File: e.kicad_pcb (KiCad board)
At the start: 2 copper layers, 69.8 x 81.6 mm, 8 parts, among them SW1 SW_Push, SW2 SW_Push, U2 MAX98357A

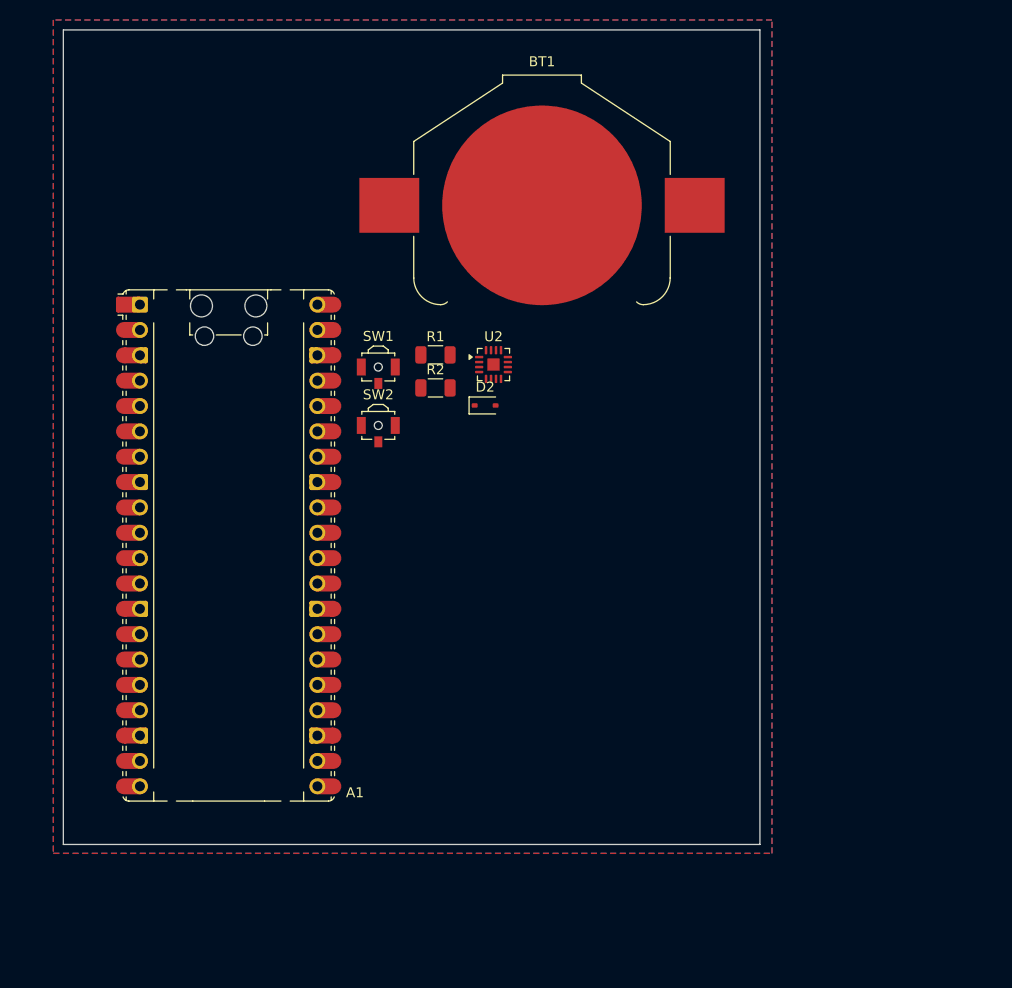
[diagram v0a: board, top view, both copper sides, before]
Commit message: i did MORE things
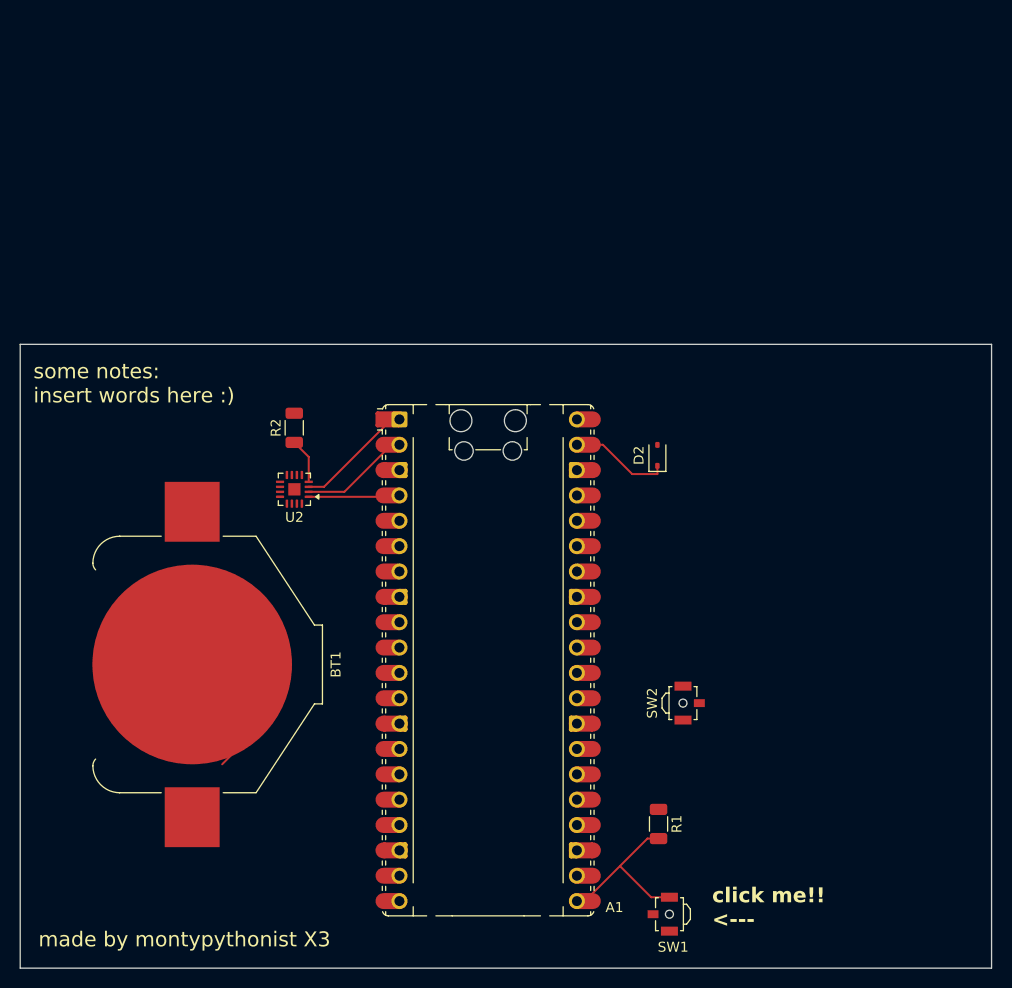
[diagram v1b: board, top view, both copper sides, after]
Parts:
- SW1: value SW_Push -> pwr
- SW2: value SW_Push -> rst
- moved SW1 61.0 mm to (159.9, 137.1), turned to -90 degrees
- moved BT1 57.8 mm to (112.9, 112.1), turned to -90 degrees
- moved R1 52.0 mm to (159.6, 128.1), turned to -90 degrees
- moved SW2 41.4 mm to (162.9, 115.9), turned to 90 degrees
- moved A1 28.4 mm to (142.6, 111.7)
- moved U2 23.5 mm to (123.2, 94.5), turned to 180 degrees
- moved D2 18.0 mm to (159.5, 91.1), turned to 90 degrees
- moved R2 14.7 mm to (123.1, 88.4), turned to 90 degrees
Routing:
- net Net-(A1-GPIO16): track 0.00 -> 16.2 mm
- net Net-(A1-GPIO0): track 0.00 -> 11.1 mm
- net Net-(A1-GPIO1): track 0.00 -> 10.2 mm
- net Net-(A1-VSYS): track 0.00 -> 9.30 mm
- net Net-(A1-GPIO2): track 0.00 -> 8.34 mm
- net GND: track 0.00 -> 8.17 mm
- net Net-(U2-GAIN_SLOT): track 0.00 -> 4.55 mm
- removed copper zone on B.Cu, net GND
- removed copper zone on F.Cu, net GND
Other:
- board size 69.8 x 81.6 mm -> 97.3 x 62.5 mm
- board text added: "click me!! <---"
- board text added: "made by montypythonist X3"
- board text added: "some notes: insert words here :)"
